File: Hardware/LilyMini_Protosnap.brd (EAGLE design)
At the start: 77.5 x 53.3 mm, 77 parts, among them Q1 ZXMP6A13F, U1 SAMD11D14A-M, U2 AP2112K-3.3V, U3 ALS-PT19, Y1 32.768kHz

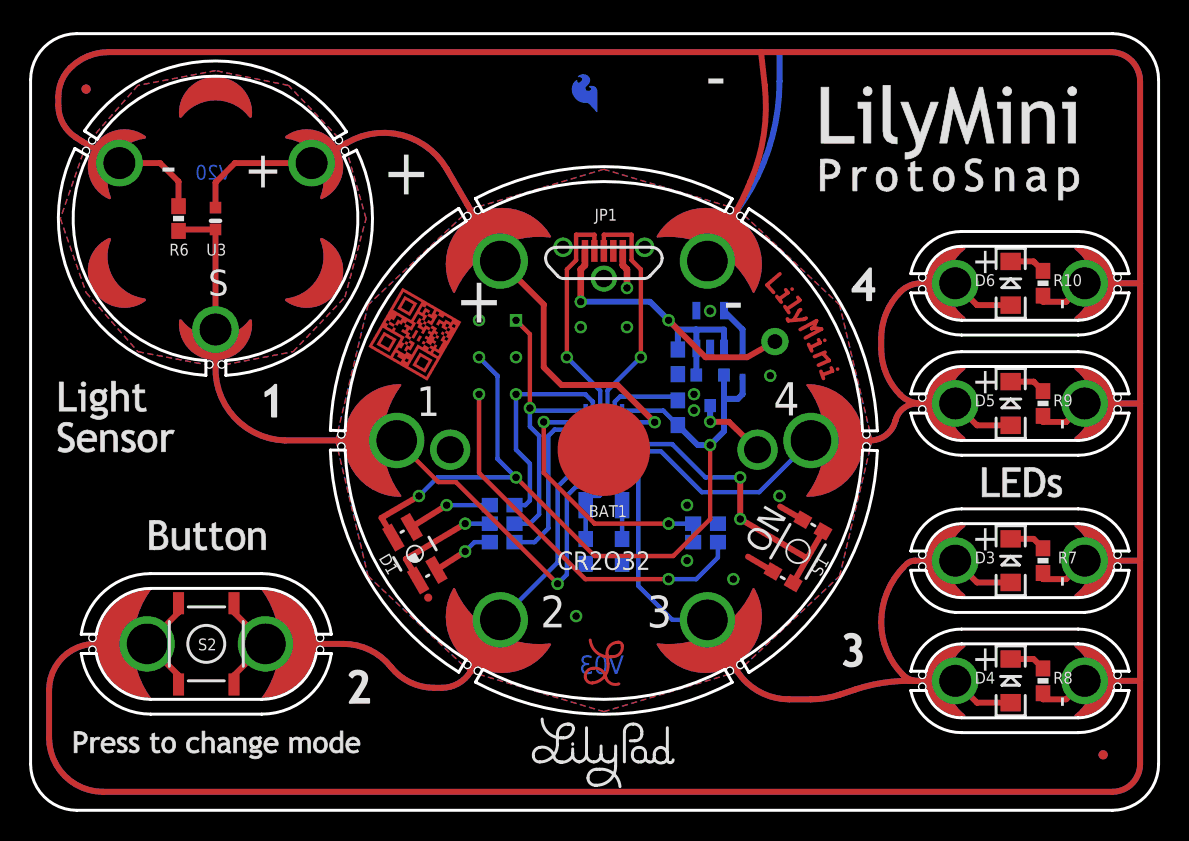
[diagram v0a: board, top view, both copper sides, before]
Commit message: Minor tweaks per board review checklist
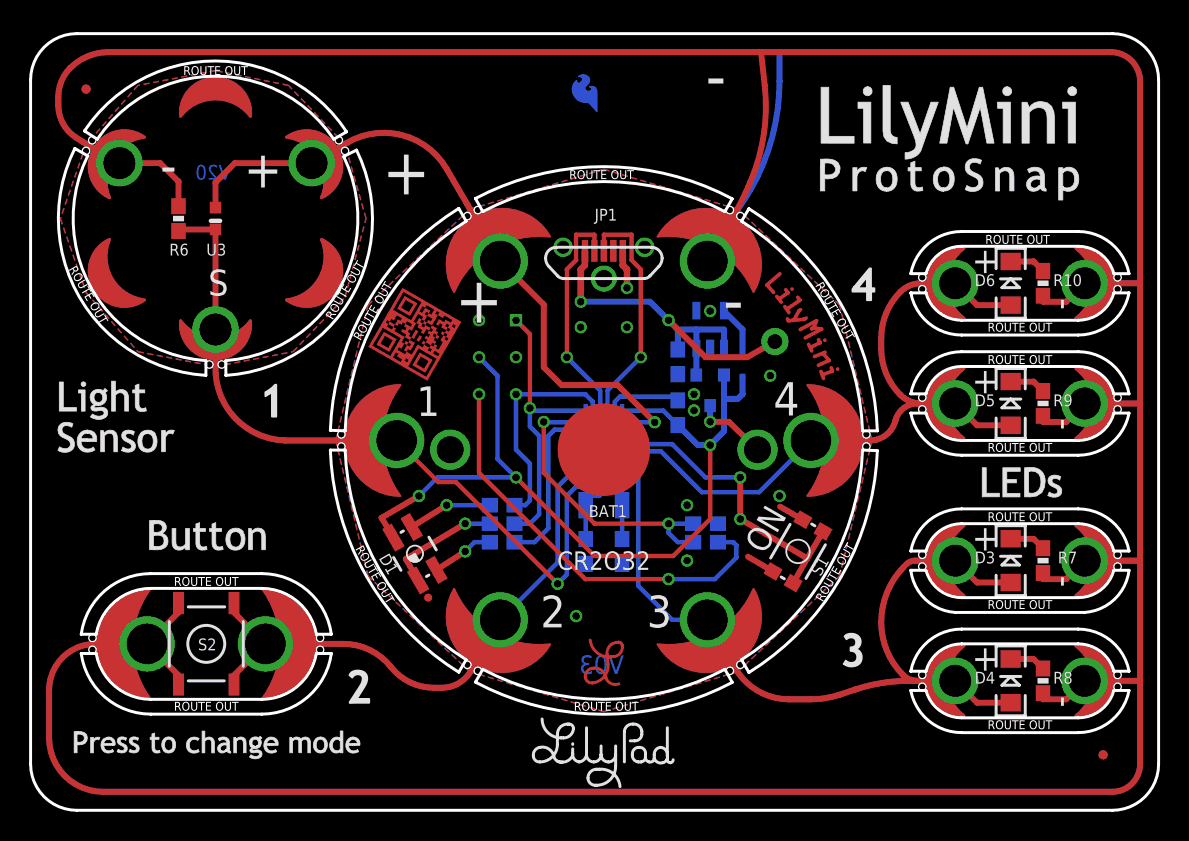
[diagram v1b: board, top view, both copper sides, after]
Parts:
- LOGO4: value (none) -> SFE_LOGO_NAME.1_INCH
- renumbered U$3 to LOGO4
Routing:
- net !RST!: track 26.5 -> 28.9 mm
- net !RST!1: track 18.7 -> 20.0 mm
- net GND: vias 12 -> 11
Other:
- board text added: "NOTE 31 MIL / 0.8MM BOARD THICKNESS"
- board text added: "ROUTE OUT"
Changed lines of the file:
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@@
 <layer number="14" name="Route14" color="1" fill="6" visible="no" active="no"/>
 <layer number="15" name="Route15" color="4" fill="6" visible="no" active="no"/>
-<layer number="16" name="Bottom" color="1" fill="1" visible="yes" active="yes"/>
-<layer number="17" name="Pads" color="2" fill="1" visible="yes" active="yes"/>
-<layer number="18" name="Vias" color="2" fill="1" visible="yes" active="yes"/>
-<layer number="19" name="Unrouted" color="6" fill="1" visible="yes" active="yes"/>
+<layer number="16" name="Bottom" color="1" fill="1" visible="no" active="yes"/>
+<layer number="17" name="Pads" color="2" fill="1" visible="no" active="yes"/>
+<layer number="18" name="Vias" color="2" fill="1" visible="no" active="yes"/>
+<layer number="19" name="Unrouted" color="6" fill="1" visible="no" active="yes"/>
 <layer number="20" name="Dimension" color="15" fill="1" visible="yes" active="yes"/>
 <layer number="21" name="tPlace" color="7" fill="1" visible="no" active="yes"/>
-<layer number="22" name="bPlace" color="7" fill="1" visible="yes" active="yes"/>
+<layer number="22" name="bPlace" color="7" fill="1" visible="no" active="yes"/>
 <layer number="23" name="tOrigins" color="15" fill="1" visible="no" active="yes"/>
-<layer number="24" name="bOrigins" color="15" fill="1" visible="yes" active="yes"/>
+<layer number="24" name="bOrigins" color="15" fill="1" visible="no" active="yes"/>
 <layer number="25" name="tNames" color="7" fill="1" visible="no" active="yes"/>
 <layer number="26" name="bNames" color="7" fill="1" visible="no" active="yes"/>
@@
 <layer number="28" name="bValues" color="7" fill="1" visible="no" active="yes"/>
 <layer number="29" name="tStop" color="7" fill="3" visible="no" active="yes"/>
-<layer number="30" name="bStop" color="7" fill="6" visible="yes" active="yes"/>
+<layer number="30" name="bStop" color="7" fill="6" visible="no" active="yes"/>
 <layer number="31" name="tCream" color="7" fill="4" visible="no" active="yes"/>
 <layer number="32" name="bCream" color="7" fill="5" visible="no" active="yes"/>
@@
 <layer number="37" name="tTest" color="7" fill="1" visible="no" active="yes"/>
 <layer number="38" name="bTest" color="7" fill="1" visible="no" active="yes"/>
-<layer number="39" name="tKeepout" color="4" fill="11" visible="yes" active="yes"/>
+<layer number="39" name="tKeepout" color="4" fill="11" visible="no" active="yes"/>
 <layer number="40" name="bKeepout" color="1" fill="11" visible="no" active="yes"/>
-<layer number="41" name="tRestrict" color="4" fill="10" visible="yes" active="yes"/>
+<layer number="41" name="tRestrict" color="4" fill="10" visible="no" active="yes"/>
 <layer number="42" name="bRestrict" color="1" fill="10" visible="no" active="yes"/>
 <layer number="43" name="vRestrict" color="2" fill="10" visible="no" active="yes"/>
@@
 <layer number="45" name="Holes" color="7" fill="1" visible="no" active="yes"/>
 <layer number="46" name="Milling" color="3" fill="1" visible="no" active="yes"/>
-<layer number="47" name="Measures" color="7" fill="1" visible="yes" active="yes"/>
+<layer number="47" name="Measures" color="7" fill="1" visible="no" active="yes"/>
 <layer number="48" name="Document" color="7" fill="1" visible="no" active="yes"/>
 <layer number="49" name="Reference" color="7" fill="1" visible="no" active="yes"/>
@@
 G 6
 B 7</text>
+<text x="38.735" y="-7.62" size="1.778" layer="51" align="center">NOTE 31 MIL / 0.8MM BOARD THICKNESS</text>
+<text x="39.52875" y="7.14375" size="0.6096" layer="20" ratio="10" align="center">ROUTE OUT</text>
+<text x="39.21125" y="43.65625" size="0.6096" layer="20" ratio="10" align="center">ROUTE OUT</text>
+<text x="67.78625" y="39.21125" size="0.6096" layer="20" ratio="10" align="center">ROUTE OUT</text>
+<text x="67.945" y="33.17875" size="0.6096" layer="20" ratio="10" align="center">ROUTE OUT</text>
+<text x="67.945" y="30.95625" size="0.6096" layer="20" ratio="10" align="center">ROUTE OUT</text>
+<text x="67.945" y="24.92375" size="0.6096" layer="20" ratio="10" align="center">ROUTE OUT</text>
+<text x="67.945" y="20.16125" size="0.6096" layer="20" ratio="10" align="center">ROUTE OUT</text>
+<text x="67.945" y="14.12875" size="0.6096" layer="20" ratio="10" align="center">ROUTE OUT</text>
+<text x="67.945" y="5.87375" size="0.6096" layer="20" ratio="10" align="center">ROUTE OUT</text>
+<text x="12.065" y="7.14375" size="0.6096" layer="20" ratio="10" align="center">ROUTE OUT</text>
+<text x="12.065" y="15.71625" size="0.6096" layer="20" ratio="10" align="center">ROUTE OUT</text>
+<text x="12.7" y="50.8" size="0.6096" layer="20" ratio="10" align="center">ROUTE OUT</text>
+<text x="23.495" y="34.29" size="0.6096" layer="20" ratio="10" rot="R60" align="center">ROUTE OUT</text>
+<text x="55.245" y="16.35125" size="0.6096" layer="20" ratio="10" rot="R60" align="center">ROUTE OUT</text>
+<text x="55.245" y="34.29" size="0.6096" layer="20" ratio="10" rot="R120" align="center">ROUTE OUT</text>
+<text x="23.65375" y="16.1925" size="0.6096" layer="20" ratio="10" rot="R120" align="center">ROUTE OUT</text>
+<text x="3.96875" y="35.40125" size="0.6096" layer="20" ratio="10" rot="R120" align="center">ROUTE OUT</text>
+<text x="21.59" y="35.71875" size="0.6096" layer="20" ratio="10" rot="R60" align="center">ROUTE OUT</text>
 </plain>
 <attributes>
@@
 <element name="JP24" library="LilyPad-Wearables" package="PETAL-SMALL-2SIDE" value="" x="63.5" y="36.195" rot="R270"/>
 <element name="JP26" library="LilyPad-Wearables" package="PETAL-SMALL-2SIDE" value="" x="63.5" y="27.94" rot="R270"/>
-<element name="U$3" library="SparkFun-Aesthetics" package="SFE_LOGO_NAME_.1" value="" x="45.72" y="44.92625" rot="MR0"/>
 <element name="U$4" library="SparkFun-Aesthetics" package="SFE_LOGO_FLAME_COPPER_EXPOSED_.1" value="" x="39.21125" y="47.625" rot="MR0"/>
 <element name="FD2" library="SparkFun-Aesthetics" package="MICRO-FIDUCIAL" value="FIDUCIALUFIDUCIAL" x="73.66" y="3.81"/>
@@
 <element name="FD3" library="SparkFun-Aesthetics" package="MICRO-FIDUCIAL" value="FIDUCIALUFIDUCIAL" x="3.81" y="49.53" rot="MR0"/>
 <element name="FD4" library="SparkFun-Aesthetics" package="MICRO-FIDUCIAL" value="FIDUCIALUFIDUCIAL" x="73.66" y="3.81" rot="MR0"/>
+<element name="LOGO4" library="SparkFun-Aesthetics" package="SFE_LOGO_NAME_.1" value="SFE_LOGO_NAME.1_INCH" x="45.72" y="44.92625" rot="MR0"/>
 </elements>
 <signals>
@@
 <contactref element="JP9" pad="P$1"/>
 <wire x1="30.7975" y1="23.1775" x2="38.1" y2="15.875" width="0.3048" layer="1"/>
-<wire x1="43.815" y1="15.875" x2="45.72" y2="15.875" width="0.3048" layer="16"/>
-<wire x1="45.72" y1="15.875" x2="47.205" y2="17.36" width="0.3048" layer="16"/>
+<wire x1="43.815" y1="15.875" x2="46.99" y2="15.875" width="0.3048" layer="16"/>
+<wire x1="46.99" y1="15.875" x2="48.475" y2="17.36" width="0.3048" layer="16"/>
 <contactref element="R5" pad="2"/>
-<wire x1="47.205" y1="17.36" x2="47.205" y2="18.415" width="0.3048" layer="16"/>
+<wire x1="48.475" y1="17.36" x2="48.475" y2="18.2" width="0.3048" layer="16"/>
+<wire x1="48.475" y1="18.2" x2="48.26" y2="18.415" width="0.3048" layer="16"/>
+<wire x1="48.26" y1="18.415" x2="47.205" y2="18.415" width="0.3048" layer="16"/>
 </signal>
 <signal name="USB5V">
@@
 <via x="45.085" y="17.145" extent="1-16" drill="0.508"/>
 <via x="51.435" y="21.59" extent="1-16" drill="0.508"/>
-<via x="48.26" y="15.875" extent="1-16" drill="0.508"/>
 <contactref element="S2" pad="4"/>
 <contactref element="S2" pad="3"/>
@@
 <wire x1="35.2425" y1="23.1775" x2="38.735" y2="19.685" width="0.3048" layer="1"/>
 <wire x1="38.735" y1="19.685" x2="43.815" y2="19.685" width="0.3048" layer="1"/>
-<wire x1="45.505" y1="18.415" x2="45.505" y2="19.685" width="0.3048" layer="16"/>
 <wire x1="45.505" y1="19.685" x2="43.815" y2="19.685" width="0.3048" layer="16"/>
 <via x="43.815" y="19.685" extent="1-16" drill="0.508"/>
+<wire x1="45.505" y1="18.415" x2="44.45" y2="18.415" width="0.3048" layer="16"/>
+<wire x1="44.45" y1="18.415" x2="43.815" y2="19.05" width="0.3048" layer="16"/>
+<wire x1="43.815" y1="19.05" x2="43.815" y2="19.685" width="0.3048" layer="16"/>
 </signal>
 <signal name="X2">
